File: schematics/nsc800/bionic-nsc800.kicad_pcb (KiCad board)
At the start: 2 copper layers, 48.3 x 71.1 mm, 10 parts, among them J1 Bionic-P135, J2 Bionic-P245, U1 NSC800N, U2 74HCT126, U3 11AA010-I/TO

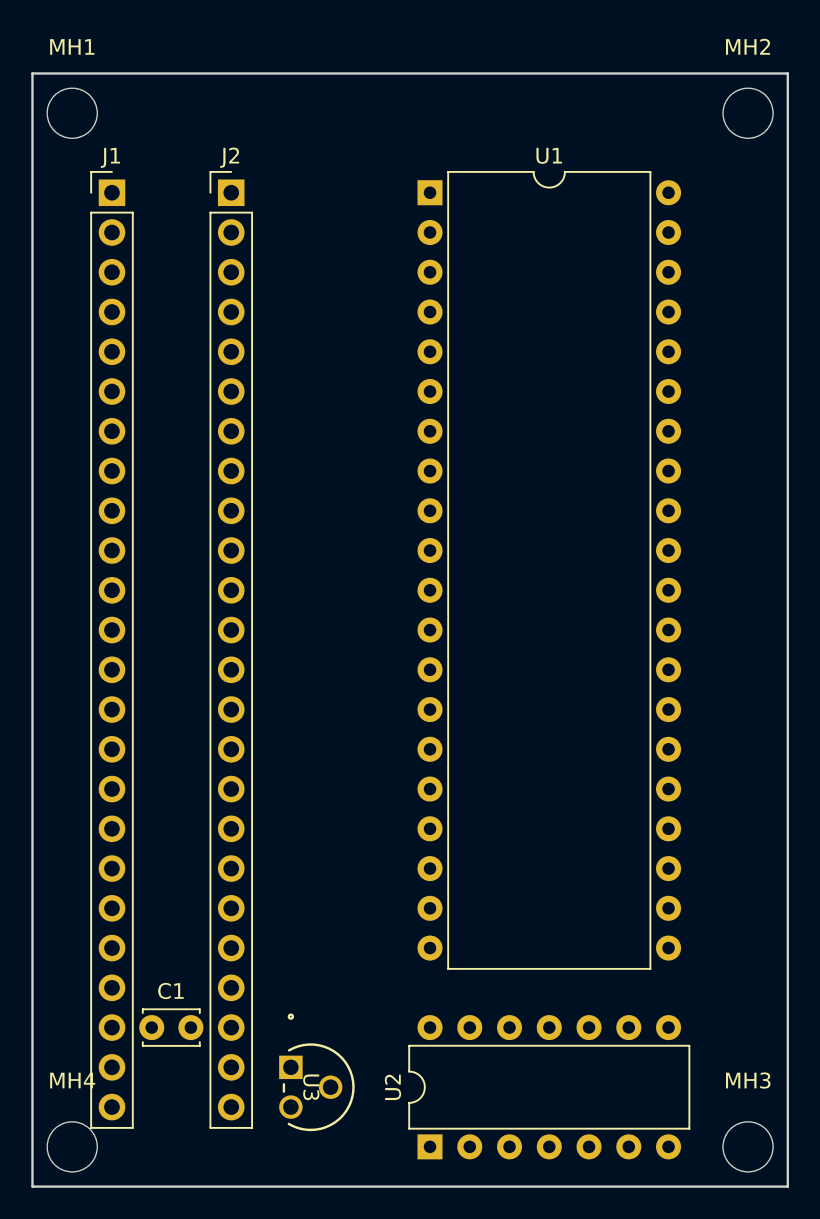
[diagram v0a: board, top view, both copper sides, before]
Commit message: [NSC800] Update schematics
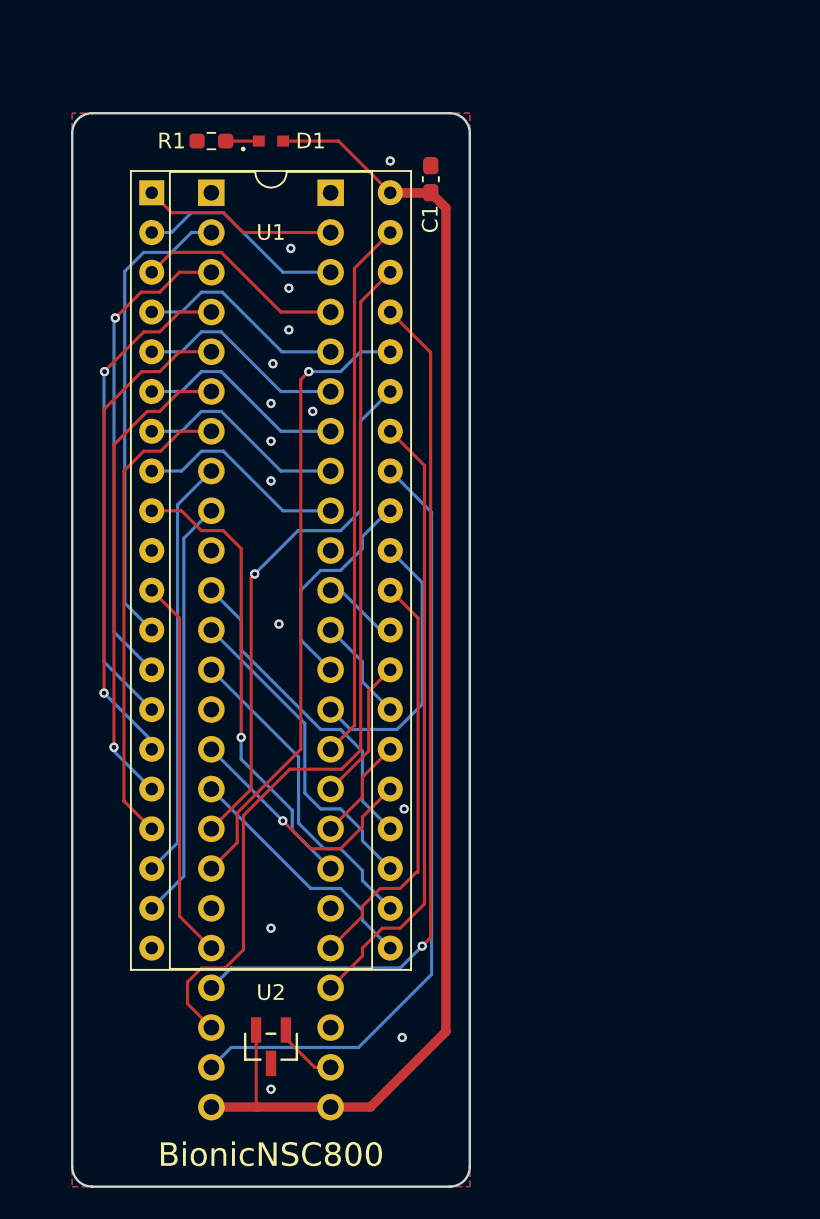
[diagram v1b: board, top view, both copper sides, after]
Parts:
- removed MH1, MH2, MH3, MH4: MountingHole_3.2mm_M3, MountingHole:MountingHole_3.2mm_M3
- removed U3: 11AA010-I/TO, microchip:TO-92_MC_MCH
- added C2: 22u, Capacitor_SMD:C_0603_1608Metric_Pad1.08x0.95mm_HandSolder, B.Cu at (123.9, 74.2)
- added D1: CSL1901UW1, 0-LocalLibrary:LED_CSL1901UW1_ROM, F.Cu at (113.7, 71.8)
- added R1: 1.6k, Resistor_SMD:R_0603_1608Metric_Pad0.98x0.95mm_HandSolder, F.Cu at (109.9, 71.8)
- C1: footprint Capacitor_THT:C_Disc_D3.4mm_W2.1mm_P2.50mm -> Capacitor_SMD:C_0603_1608Metric_Pad1.08x0.95mm_HandSolder
- J1: footprint connector:Bionic-P135_Vertical -> 0-LocalLibrary:Bionic-P135_Vertical; moved to B.Cu
- J2: footprint connector:Bionic-P245_Vertical -> 0-LocalLibrary:Bionic-P245_Vertical; moved to B.Cu
- U1: footprint Package_DIP:DIP-40_W15.24mm -> 0-LocalLibrary:DIP-40_W15.24mm_Socket
- U2: value 74HCT126 -> 11AA010-I/TT; footprint Package_DIP:DIP-14_W7.62mm -> 0-LocalLibrary:SOT-23_MC_MCH-M
- moved C1 57.1 mm to (123.9, 74.2), turned to 90 degrees
- moved U1 17.8 mm to (106.1, 75.1)
- moved U2 12.0 mm to (113.7, 129.6), turned to 180 degrees
- moved J2 6.35 mm to (117.5, 75.1), turned to 180 degrees
- moved J1 6.35 mm to (109.9, 75.1), turned to 180 degrees
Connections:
- J2 pad 37: unconnected-(J2-P41-Pad37) -> /P41
- U1 pad 11: Net-(U1-XIN) -> /P50
- U1 pad 21: /P43 -> /P35
- U1 pad 22: /P30 -> /P32
- U1 pad 24: /P32 -> /P30
- U1 pad 25: /P42 -> /P34
- U1 pad 26: /P54 -> /P46
- U1 pad 27: /P35 -> /P41
- U1 pad 29: /P34 -> /P40
- U1 pad 30: /P40 -> /P54
- U1 pad 31: /P51 -> /P43
- U1 pad 32: /P50 -> /P42
- U1 pad 33: Net-(U1-~{RESETIN}) -> /P53
- U1 pad 37: unconnected-(U1-RESETO-Pad37) -> /P51
- U2 pad 1: VCC -> Net-(J2-P57)
- U2 pad 2: /P46 -> VCC
- U2 pad 3: Net-(U1-XIN) -> GND
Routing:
- net VCC: track 0.00 -> 89.5 mm
- net /P52: track 0.00 -> 57.1 mm
- net /P51: track 0.00 -> 56.4 mm, vias 0 -> 1
- net /P53: track 0.00 -> 49.8 mm
- net /P37: track 0.00 -> 40.1 mm, vias 0 -> 1
- net /P55: track 0.00 -> 39.6 mm
- net /P44: track 0.00 -> 34.6 mm
- net /P36: track 0.00 -> 34.3 mm, vias 0 -> 1
- net /P13: track 0.00 -> 31.4 mm, vias 0 -> 1
- net /P12: track 0.00 -> 31.3 mm, vias 0 -> 1
- net /P11: track 0.00 -> 30.9 mm, vias 0 -> 1
- net /P14: track 0.00 -> 30.6 mm, vias 0 -> 1
- net /P15: track 0.00 -> 30.2 mm
- net /P10: track 0.00 -> 30.2 mm
- net /P47: track 0.00 -> 30.2 mm, vias 0 -> 1
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- added copper zone on B.Cu, net GND
- added copper zone on F.Cu, net GND
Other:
- board size 48.3 x 71.1 mm -> 25.4 x 68.6 mm
- board text added: "BionicNSC800"
- board text added: "JLCJLCJLCJLC"
- board text added: "Rev. 3"
